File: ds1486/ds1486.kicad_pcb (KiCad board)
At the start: 4 copper layers, 30.4 x 43.9 mm, 55 parts, among them J1 DBG, J2 DBG1-16, J3 DBG17-32, J4 DS1-16, J5 DS17-32, U1 RP2040, U3 AMS1117-3.3, U4 SN74LVC8T245, U5 SN74LVC1G00DRL, U6 YSN8010SJ, U7 SN74LVC1G00DRL, U8 W25Q16JVSS, Y2 E3SB12E00004EE

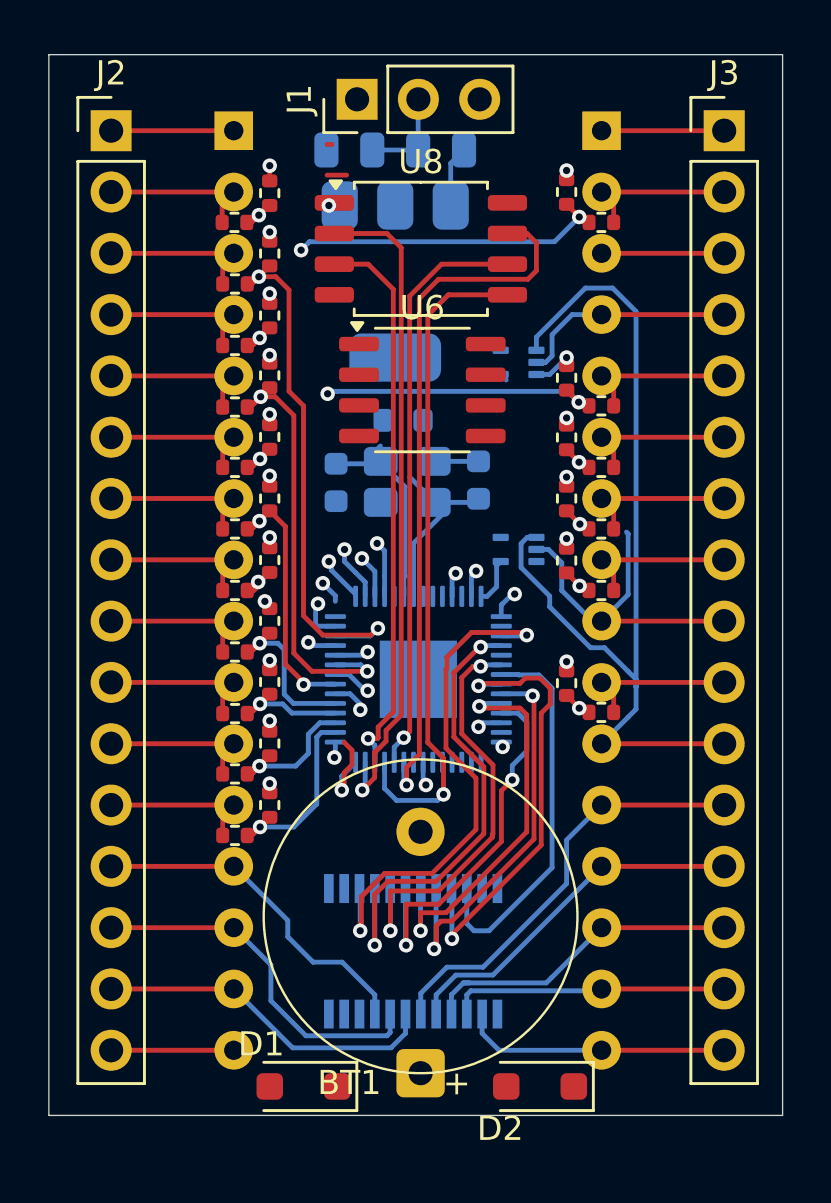
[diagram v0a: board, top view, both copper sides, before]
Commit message: Fully routed.
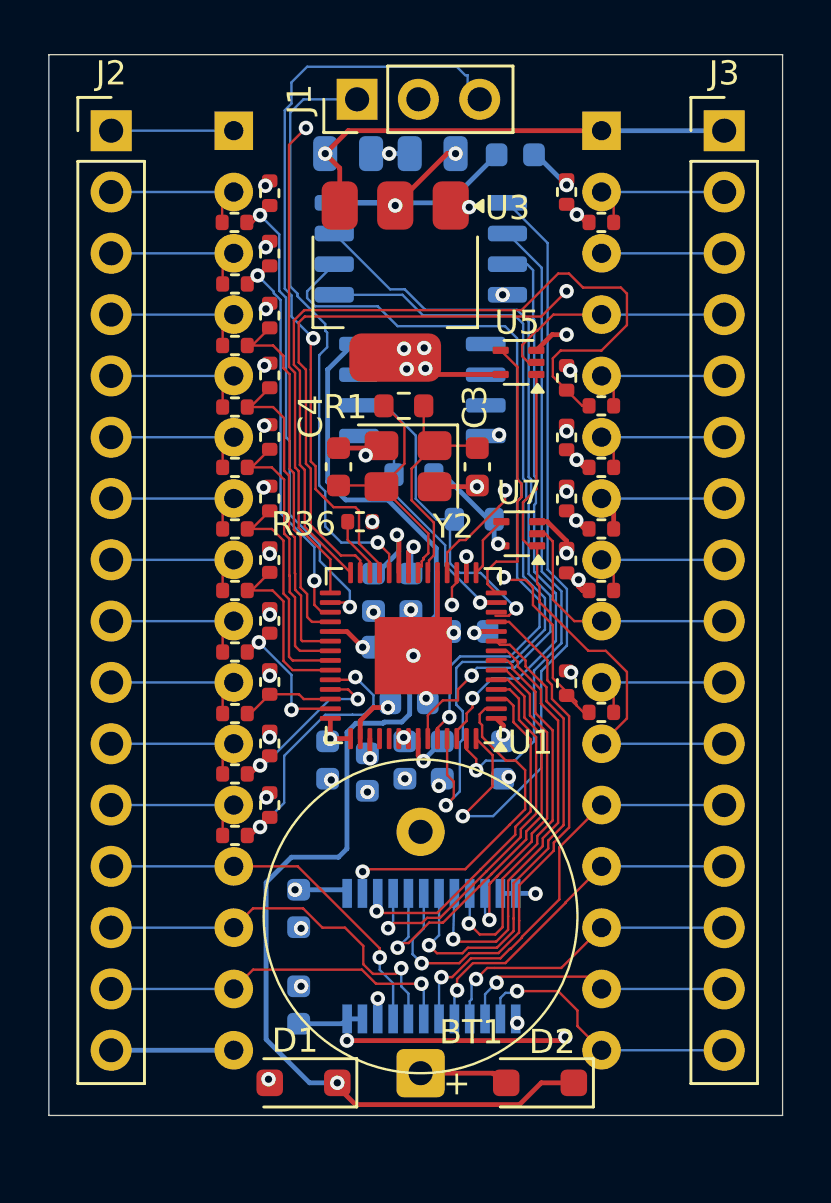
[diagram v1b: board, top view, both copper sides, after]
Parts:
- added C10: 100n, Capacitor_SMD:C_0603_1608Metric, B.Cu at (121.5, 84.2)
- added C11: 1u, Capacitor_SMD:C_0603_1608Metric, B.Cu at (119.0, 87.2)
- added C12: 1u, Capacitor_SMD:C_0603_1608Metric, B.Cu at (117.3, 90.1)
- added C13: 100n, Capacitor_SMD:C_0603_1608Metric, B.Cu at (117.5, 82.6)
- added C14: 100n, Capacitor_SMD:C_0603_1608Metric, B.Cu at (120.4, 89.6)
- added C15: 100n, Capacitor_SMD:C_0603_1608Metric, B.Cu at (114.5, 95.7)
- added C16: 100n, Capacitor_SMD:C_0603_1608Metric, B.Cu at (114.5, 99.7)
- added C17: 100n, Capacitor_SMD:C_0603_1608Metric, B.Cu at (123.4, 64.5)
- added C5: 100n, Capacitor_SMD:C_0603_1608Metric, B.Cu at (118.8, 89.6)
- added C6: 100n, Capacitor_SMD:C_0603_1608Metric, B.Cu at (115.7, 89.6)
- added C7: 100n, Capacitor_SMD:C_0603_1608Metric, B.Cu at (118.3, 84.9)
- added C8: 100n, Capacitor_SMD:C_0603_1608Metric, B.Cu at (119.1, 82.6)
- added C9: 100n, Capacitor_SMD:C_0603_1608Metric, B.Cu at (122.9, 89.6)
- added R36: 10k, Resistor_SMD:R_0402_1005Metric, F.Cu at (117.0, 79.7)
- added R37: 4k7, Resistor_SMD:R_0603_1608Metric, B.Cu at (121.7, 79.6)
- added R38: 4k7, Resistor_SMD:R_0603_1608Metric, B.Cu at (119.2, 77.8)
- C3, C4, R1, U1, U3, U5, U7, Y2: moved to F.Cu
- U6, U8: moved to B.Cu
- moved C3 5.89 mm to (121.8, 77.4)
- moved C4 5.83 mm to (116.1, 77.4)
- moved C1 3.85 mm to (116.5, 64.5), turned to 0 degrees
- moved C2 3.45 mm to (120.0, 64.5), turned to 180 degrees
- moved U1 1.00 mm to (119.2, 85.2), turned to 180 degrees
- moved U4 0.78 mm to (120.0, 97.7)
- moved U7 0.65 mm to (123.6, 80.2)
- moved Y2 0.65 mm to (119.0, 77.4), turned to 180 degrees
- moved R1 0.60 mm to (118.8, 74.9), turned to 180 degrees
- moved D1 0.15 mm to (114.7, 103.0)
- moved D2 0.15 mm to (124.5, 103.0)
- turned U6 to 180 degrees
- turned U8 to 180 degrees
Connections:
- U1 pad 11: /AC12 -> /DQC7
- U1 pad 12: /AC14 -> /SCL
- U1 pad 13: /AC16 -> /SDA
- U1 pad 14: /AC15 -> /CE_WE
- U1 pad 15: /AC13 -> /CE_OE
- U1 pad 16: /AC8 -> /AC10
- U1 pad 17: /AC9 -> /AC11
- U1 pad 18: /AC11 -> /AC9
- U1 pad 19: unconnected-(U1-TESTEN-Pad19) -> GND
- U1 pad 2: /AC0 -> /D_DIR
- U1 pad 23: Net-(U1-DVDD-Pad23) -> +1V1
- U1 pad 26: unconnected-(U1-RUN-Pad26) -> /RUN
- U1 pad 27: /AC10 -> /AC8
- U1 pad 28: /CE_OE -> /AC13
- U1 pad 29: /CE_WE -> /AC15
- U1 pad 3: /AC1 -> /DQC0
- U1 pad 30: /SCL -> /AC16
- U1 pad 31: /DQC0 -> /AC14
- U1 pad 32: /DQC1 -> /AC12
- U1 pad 34: /DQC2 -> /AC7
- U1 pad 35: /DQC3 -> /AC6
- U1 pad 36: /DQC4 -> /AC5
- U1 pad 37: /DQC5 -> /AC4
- U1 pad 38: /DQC6 -> /AC0
- U1 pad 39: /DQC7 -> /AC1
- U1 pad 4: /AC2 -> /DQC1
- U1 pad 40: GND -> /AC2
- U1 pad 41: /SDA -> /AC3
- U1 pad 43: unconnected-(U1-ADC_AVDD-Pad43) -> +3V3
- U1 pad 44: unconnected-(U1-VREG_IN-Pad44) -> +3V3
- U1 pad 45: unconnected-(U1-VREG_VOUT-Pad45) -> +1V1
- U1 pad 48: unconnected-(U1-USB_VDD-Pad48) -> +3V3
- U1 pad 5: /AC3 -> /DQC2
- U1 pad 50: Net-(U1-DVDD-Pad23) -> +1V1
- U1 pad 6: /AC4 -> /DQC3
- U1 pad 7: /AC5 -> /DQC4
- U1 pad 8: /AC6 -> /DQC5
- U1 pad 9: /AC7 -> /DQC6
- U4 pad 2: unconnected-(U4-DIR-Pad2) -> /D_DIR
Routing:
- net +5V: track 7.61 -> 72.8 mm, vias 0 -> 3
- net +3V3: track 3.26 -> 67.3 mm, vias 4 -> 17
- net /VRTC: track 0.00 -> 51.7 mm, vias 0 -> 1
- net /SWD: track 1.02 -> 31.6 mm
- net /QSPI_SS: track 4.70 -> 33.0 mm
- net /SWCLK: track 0.00 -> 24.9 mm, vias 0 -> 1
- net +1V1: track 0.00 -> 18.9 mm, vias 0 -> 3
- net /AC8: track 17.6 -> 35.8 mm
- net /CE_: track 38.5 -> 23.5 mm
- net /D_DIR: track 0.00 -> 14.5 mm, vias 0 -> 1
- net /SCL: track 0.00 -> 13.8 mm, vias 0 -> 1
- net /AC13: track 21.1 -> 34.1 mm, vias 3 -> 0
- net /SDA: track 0.00 -> 10.7 mm, vias 0 -> 1
- net /CE_WE: track 1.54 -> 11.7 mm, vias 1 -> 0
- net GND: track 22.7 -> 31.8 mm, vias 19 -> 39
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- added copper zone on In1.Cu, net +3V3
